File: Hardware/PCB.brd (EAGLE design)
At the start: 170.2 x 111.2 mm, 103 parts, among them IC1 BD5229G-TR, IC4 XC6220A331MR-G, J1 FH34SRJ-24S-0.5SH_99_, J3 QWIIC_RIGHT_ANGLE, J4 112A-TAAR-R03_ATTEND, Q1 20V/4.2A/52mΩ/1.4W, Q2 20V/4.2A/52mΩ/1.4W, Q3 SI1308EDL-T1-GE3, U1 W25Q512JVEIQ, U2 ESP32-C6-WROOM-1-N8, U3 DS3231SN#, U4 MAX17048G+T10

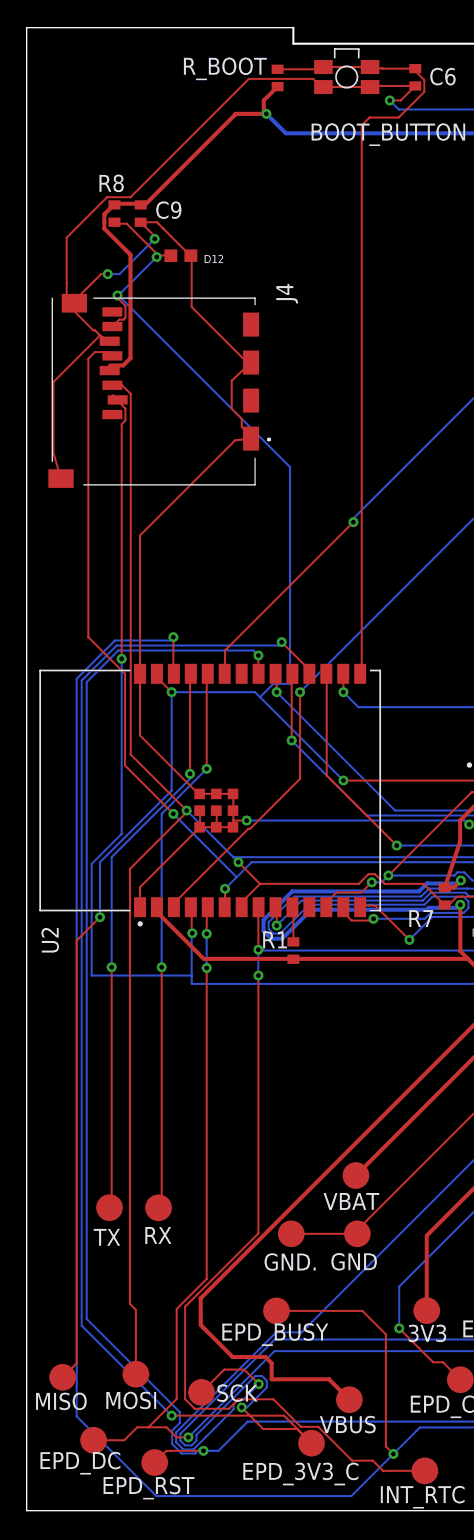
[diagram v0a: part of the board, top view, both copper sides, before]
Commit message: add files
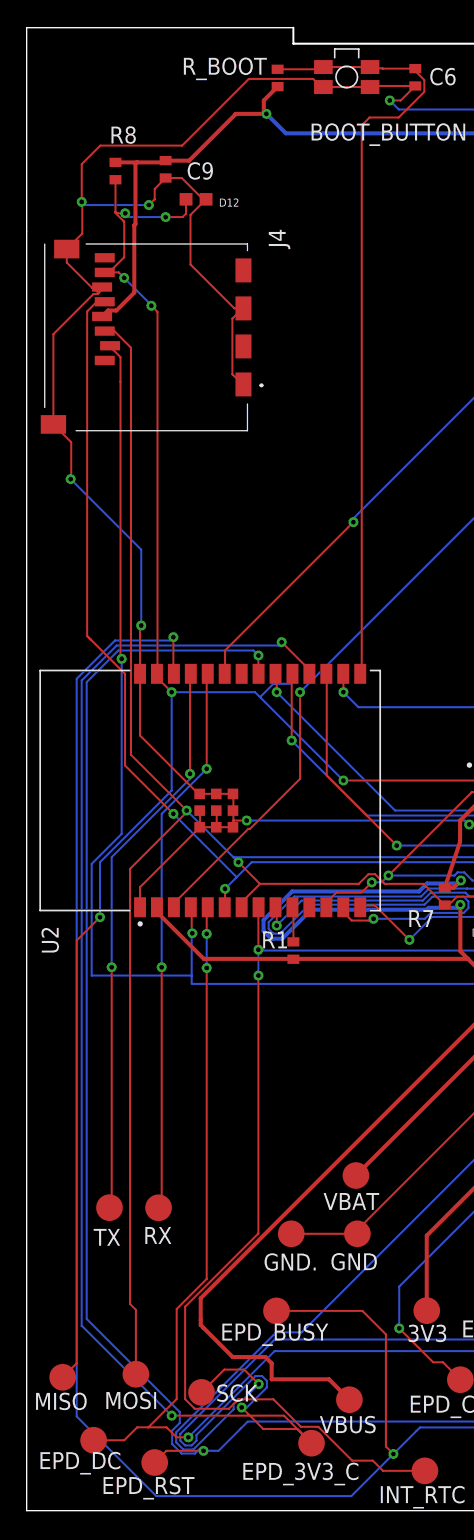
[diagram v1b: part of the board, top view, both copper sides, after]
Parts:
- moved D12 4.38 mm to (12.7, 98.3)
- moved J4 4.10 mm to (5.86, 95.0)
- moved C9 3.81 mm to (10.4, 100.6)
- moved R8 3.19 mm to (6.66, 100.5)
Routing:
- net GND: track 731.2 -> 726.2 mm, vias 8 -> 10
- net MOSI: track 203.7 -> 208.0 mm
- net SCK: track 234.7 -> 238.0 mm
- net 3V3: track 479.0 -> 475.9 mm
- net SS_SD: track 99.3 -> 102.5 mm
- net MISO: track 132.8 -> 132.6 mm, vias 5 -> 7
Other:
- outline, holes or cut-outs redrawn
